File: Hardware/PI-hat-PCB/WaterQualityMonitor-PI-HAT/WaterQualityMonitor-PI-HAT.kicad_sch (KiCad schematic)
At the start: 37 parts

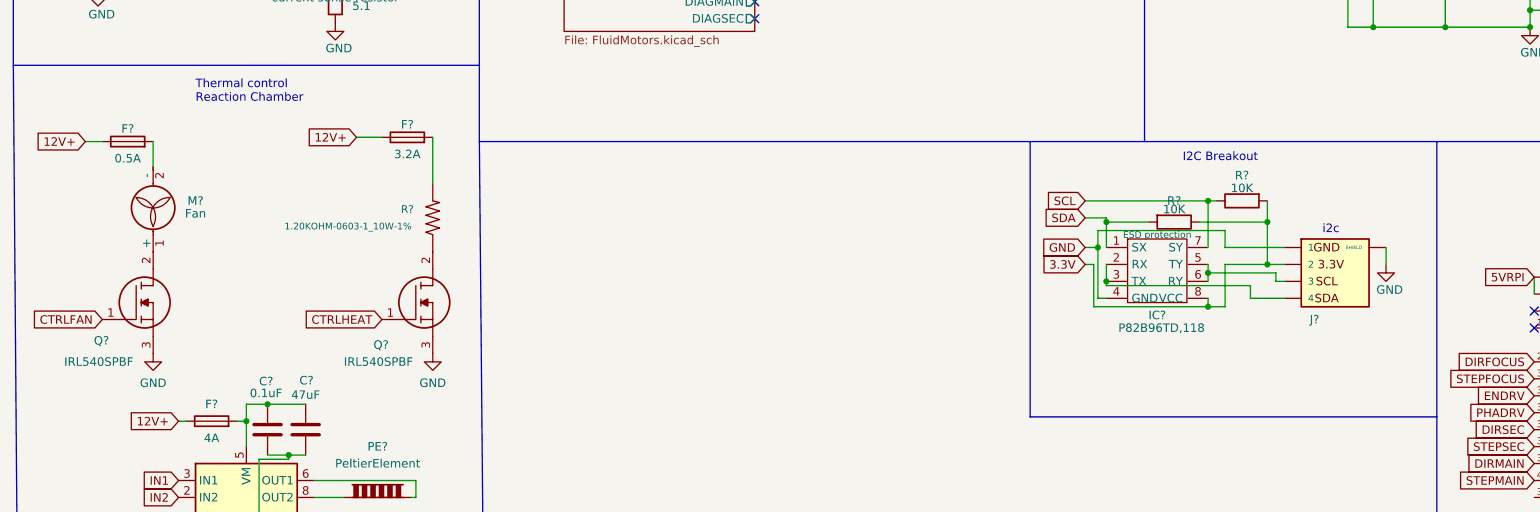
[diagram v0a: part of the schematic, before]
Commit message: enhanced layout
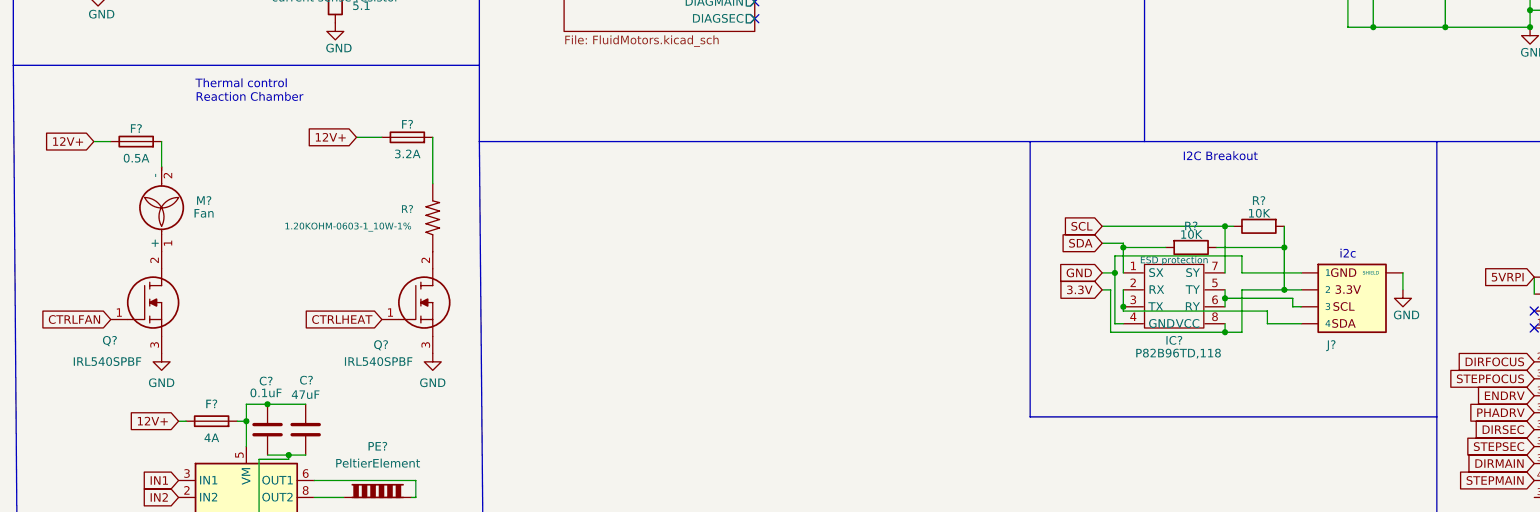
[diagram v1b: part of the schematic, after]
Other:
- moved on the sheet: F?, IC?, J?, M?, Q?, R?
